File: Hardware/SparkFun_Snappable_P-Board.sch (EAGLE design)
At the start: 128 parts

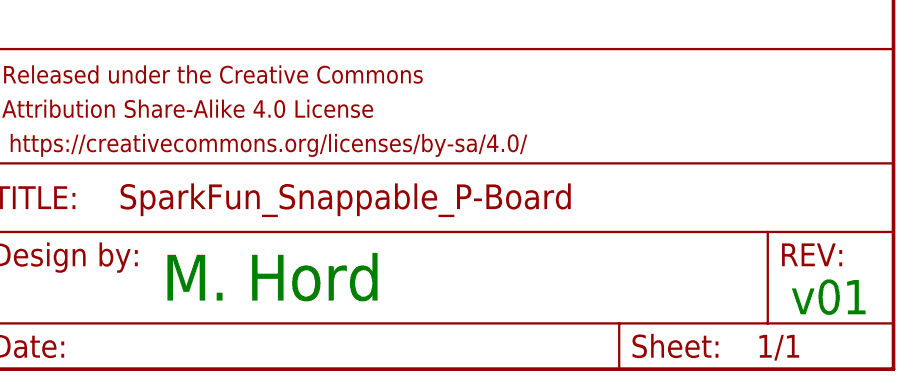
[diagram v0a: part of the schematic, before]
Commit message: Ready for protos
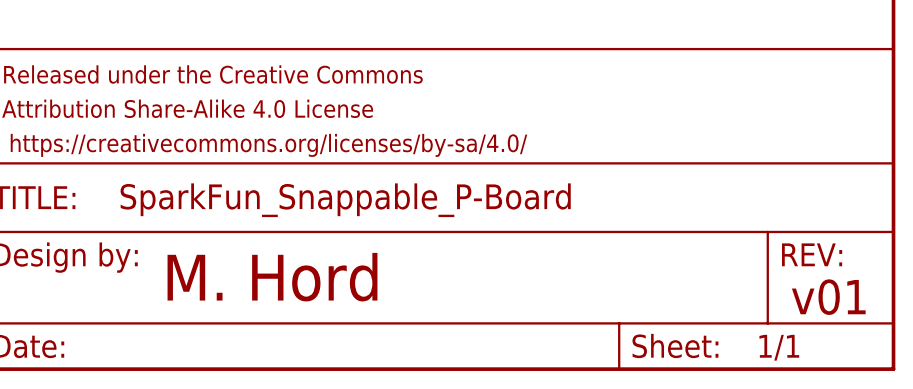
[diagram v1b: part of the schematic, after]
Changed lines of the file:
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@@
 <sheet>
 <plain>
-<text x="350.52" y="7.62" size="5.08" layer="91">M. Hord</text>
-<text x="420.37" y="6.096" size="3.81" layer="91">v01</text>
+<text x="350.52" y="7.62" size="5.08" layer="94">M. Hord</text>
+<text x="420.37" y="6.096" size="3.81" layer="94">v01</text>
 </plain>
 <instances>

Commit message: Fixed logo line thickness
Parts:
- JP1, JP10, JP100, JP101, JP102, JP103, JP104, JP105, JP106, JP107, JP108, JP109, JP11, JP110, JP111, JP112, JP113, JP114, JP115, JP116, JP117, JP118, JP119, JP12, JP120, JP121, JP122, JP123, JP124, JP125, JP13, JP14, JP15, JP16, JP17, JP18, JP19, JP2, JP20, JP21, JP22, JP23, JP24, JP25, JP26, JP27, JP28, JP29, JP3, JP30, JP31, JP32, JP33, JP34, JP35, JP36, JP37, JP38, JP39, JP4, JP40, JP41, JP42, JP43, JP44, JP45, JP46, JP47, JP48, JP49, JP5, JP50, JP51, JP52, JP53, JP54, JP55, JP56, JP57, JP58, JP59, JP6, JP60, JP61, JP62, JP63, JP64, JP65, JP66, JP67, JP68, JP69, JP7, JP70, JP71, JP72, JP73, JP74, JP75, JP76, JP77, JP78, JP79, JP8, JP80, JP81, JP82, JP83, JP84, JP85, JP86, JP87, JP88, JP89, JP9, JP90, JP91, JP92, JP93, JP94, JP95, JP96, JP97, JP98, JP99: value M10NO_SILK_PTH_FEMALE -> (none)
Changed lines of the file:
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@@
 <layer number="56" name="wert" color="7" fill="1" visible="no" active="no"/>
 <layer number="57" name="tCAD" color="7" fill="1" visible="no" active="no"/>
+<layer number="59" name="tCarbon" color="7" fill="1" visible="no" active="no"/>
+<layer number="60" name="bCarbon" color="7" fill="1" visible="no" active="no"/>
 <layer number="90" name="Modules" color="5" fill="1" visible="yes" active="yes"/>
 <layer number="91" name="Nets" color="2" fill="1" visible="yes" active="yes"/>
@@
 <layer number="127" name="_tValues" color="7" fill="1" visible="yes" active="yes"/>
 <layer number="128" name="_bValues" color="7" fill="1" visible="yes" active="yes"/>
+<layer number="129" name="Mask" color="7" fill="1" visible="yes" active="yes"/>
 <layer number="131" name="tAdjust" color="7" fill="1" visible="yes" active="yes"/>
 <layer number="132" name="bAdjust" color="7" fill="1" visible="yes" active="yes"/>
@@
 <layer number="223" name="223bmp" color="24" fill="1" visible="no" active="no"/>
 <layer number="224" name="224bmp" color="25" fill="1" visible="no" active="no"/>
+<layer number="225" name="225bmp" color="7" fill="1" visible="yes" active="yes"/>
+<layer number="226" name="226bmp" color="7" fill="1" visible="yes" active="yes"/>
+<layer number="227" name="227bmp" color="7" fill="1" visible="yes" active="yes"/>
+<layer number="228" name="228bmp" color="7" fill="1" visible="yes" active="yes"/>
+<layer number="229" name="229bmp" color="7" fill="1" visible="yes" active="yes"/>
+<layer number="230" name="230bmp" color="7" fill="1" visible="yes" active="yes"/>
+<layer number="231" name="231bmp" color="7" fill="1" visible="yes" active="yes"/>
 <layer number="248" name="Housing" color="7" fill="1" visible="yes" active="yes"/>
 <layer number="249" name="Edge" color="7" fill="1" visible="yes" active="yes"/>
@@
 <layer number="251" name="SMDround" color="12" fill="11" visible="no" active="no"/>
 <layer number="254" name="cooling" color="7" fill="1" visible="yes" active="yes"/>
+<layer number="255" name="routoute" color="7" fill="1" visible="yes" active="yes"/>
 </layers>
 <schematic xreflabel="%F%N/%S" xrefpart="1_/%S.%C%R">
